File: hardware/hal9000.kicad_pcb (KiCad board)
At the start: 2 copper layers, 53.6 x 59.9 mm, 17 parts

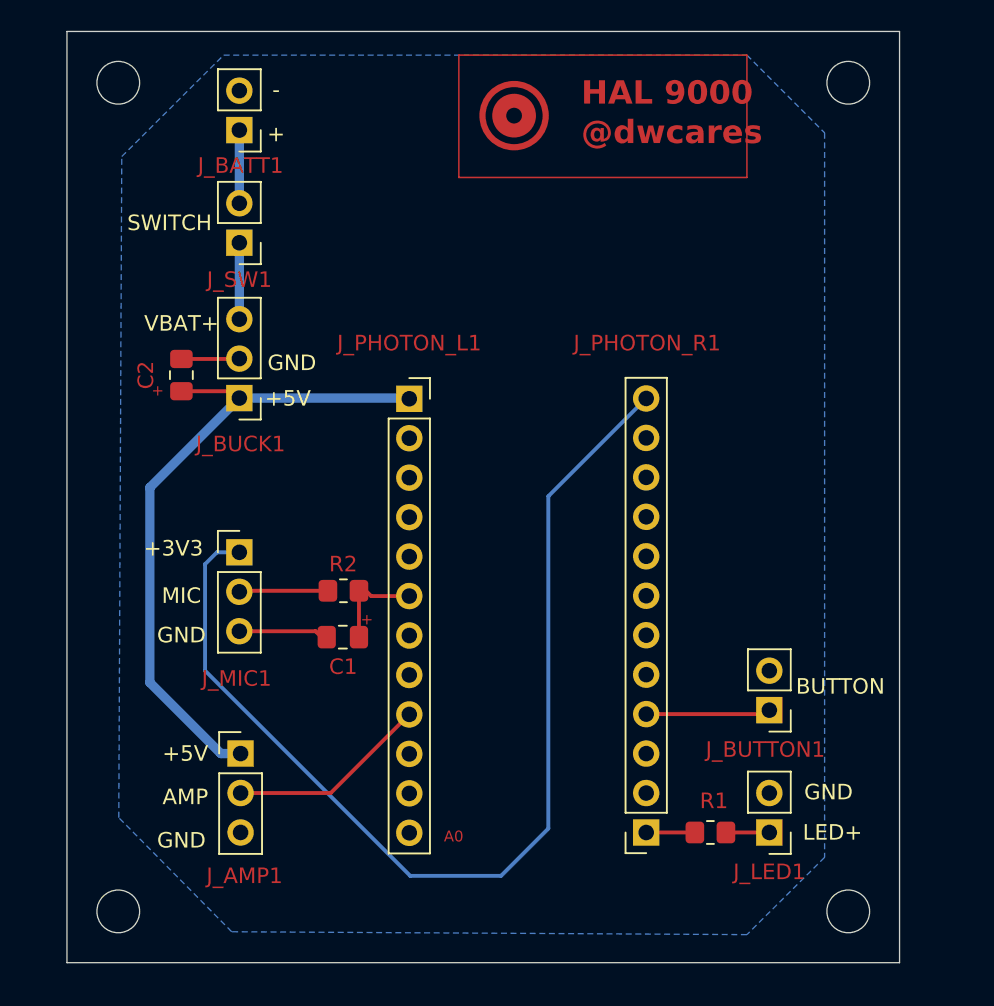
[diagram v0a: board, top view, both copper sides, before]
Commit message: hw: reva2 kicad files
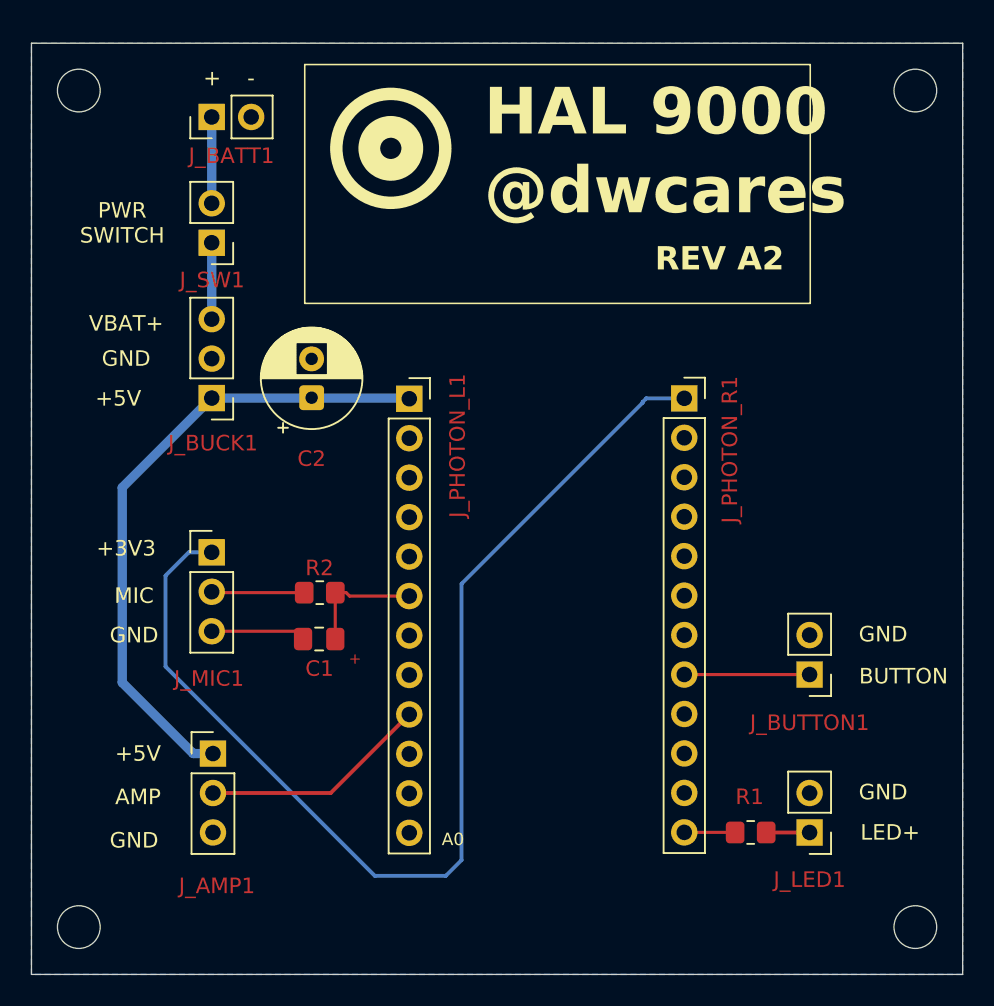
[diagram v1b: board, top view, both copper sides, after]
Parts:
- C2: footprint Capacitor_SMD:C_0805_2012Metric_Pad1.18x1.45mm_HandSolder -> Capacitor_THT:CP_Radial_D6.3mm_P2.50mm
- moved J_PHOTON_R1 28.1 mm to (160.6, 86.9), turned to 0 degrees
- moved C2 8.51 mm to (136.7, 86.8)
- moved ? 4.43 mm to (175.5, 120.9)
- moved ? 4.35 mm to (175.5, 67.0)
- moved J_BUTTON1 3.46 mm to (168.7, 104.6)
- moved ? 2.73 mm to (121.7, 120.9)
- moved J_LED1 2.59 mm to (168.7, 114.8)
- moved R1 2.59 mm to (164.9, 114.8)
- moved ? 2.59 mm to (121.7, 67.0)
- moved J_BATT1 1.97 mm to (130.2, 68.8), turned to 90 degrees
- moved J_AMP1 1.78 mm to (130.3, 109.7)
- moved J_BUCK1 1.78 mm to (130.2, 86.8)
- moved J_MIC1 1.78 mm to (130.2, 96.8)
- moved J_SW1 1.78 mm to (130.2, 76.8)
- moved C1 1.53 mm to (137.1, 102.4)
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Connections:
- J_BUTTON1 pad 1: Net-(J_BUTTON1-Pin_1) -> /D3
- J_PHOTON_R1 pad 1: Net-(J_PHOTON_R1-Pin_1) -> +3V3
- J_PHOTON_R1 pad 12: +3V3 -> /D0
- J_PHOTON_R1 pad 4: Net-(J_BUTTON1-Pin_1) -> unconnected-(J_PHOTON_R1-Pin_4-Pad4)
- J_PHOTON_R1 pad 8: unconnected-(J_PHOTON_R1-Pin_8-Pad8) -> /D3
- R1 pad 2: Net-(J_PHOTON_R1-Pin_1) -> /D0
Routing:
- net /D3: track 0.00 -> 8.18 mm
- net Net-(J_BUTTON1-Pin_1): track 8.03 -> 0.00 mm
- net Net-(J_PHOTON_R1-Pin_1): track 4.04 -> 0.00 mm
- net /D0: track 0.00 -> 3.73 mm
- net GND: track 9.63 -> 6.47 mm
- net +3V3: track 68.5 -> 71.6 mm
- net /A6: track 6.37 -> 8.28 mm
- net /A3: track 13.0 -> 14.7 mm
- net +5V: track 43.3 -> 41.8 mm
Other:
- board size 53.6 x 59.9 mm -> 59.9 x 59.9 mm
- board text added: "PWR SWITCH"
- board text added: "REV A2"
- board text removed: "SWITCH"
